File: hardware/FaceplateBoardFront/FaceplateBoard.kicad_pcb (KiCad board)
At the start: 2 copper layers, 33 x 66.5 mm, 20 parts, among them SW1 Mode_Encoder, SW2 Color_Encoder

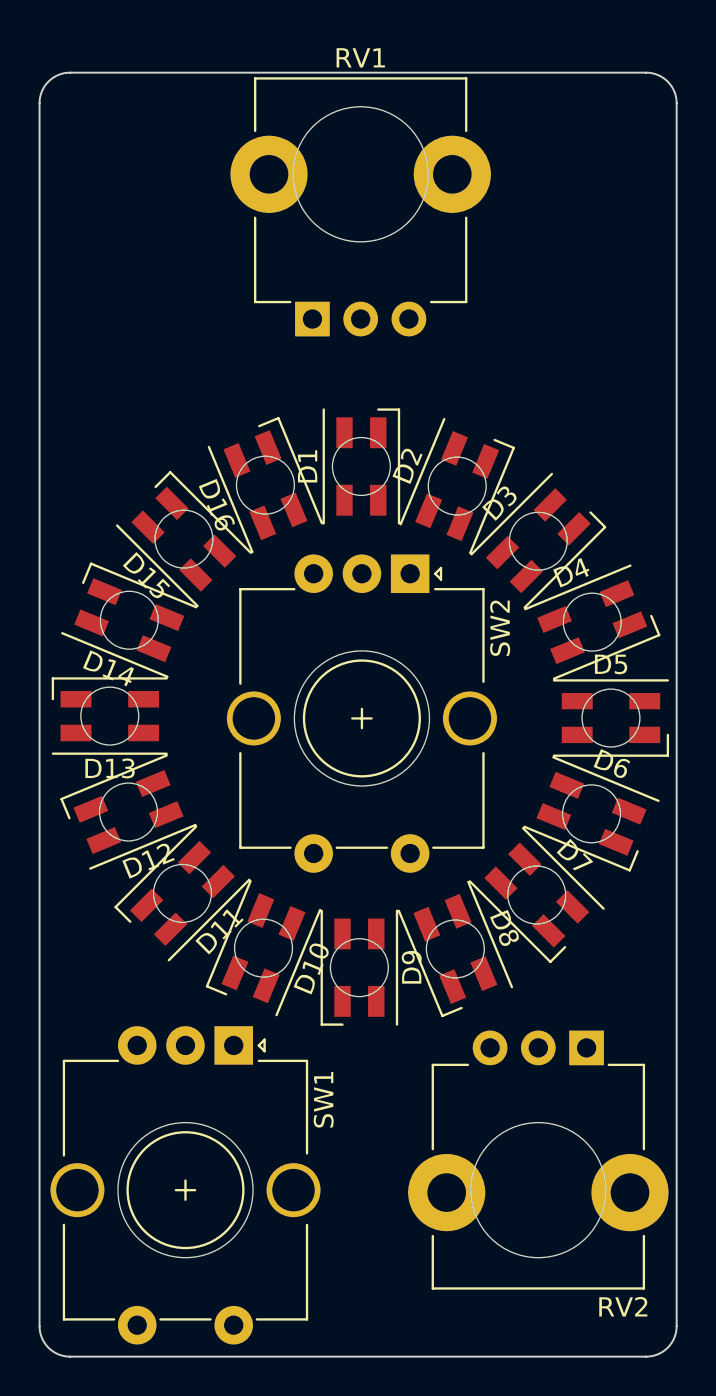
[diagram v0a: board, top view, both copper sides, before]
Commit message: After PCB v2
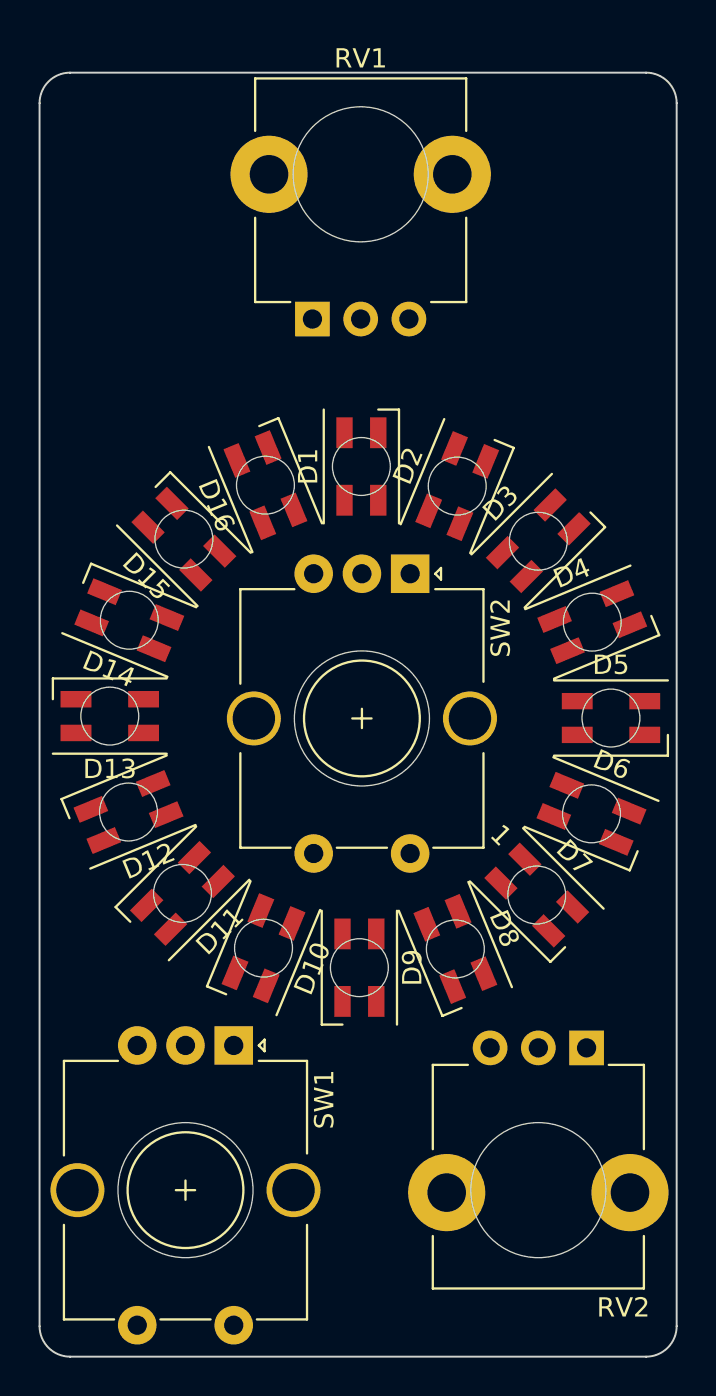
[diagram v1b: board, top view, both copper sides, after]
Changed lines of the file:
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@@
     (tags "LED RGB NeoPixel Mini")
     (attr smd)
-    (fp_text reference D16 (at 0 -2.75 112.5) (layer F.SilkS)
-      (effects (font (size 1 1) (thickness 0.15)))
-    )
-    (fp_text value WS2812B (at 0 3.25 112.5) (layer F.Fab)
+    (fp_text reference D16 (at 0.000001 -2.75 112.5) (layer F.SilkS)
+      (effects (font (size 1 1) (thickness 0.15)))
+    )
+    (fp_text value WS2812B (at 0 3.249999 112.5) (layer F.Fab)
       (effects (font (size 1 1) (thickness 0.15)))
     )
@@
     (tags "LED RGB NeoPixel Mini")
     (attr smd)
-    (fp_text reference D2 (at 0 -2.75 67.5) (layer F.SilkS)
-      (effects (font (size 1 1) (thickness 0.15)))
-    )
-    (fp_text value WS2812B (at 0 3.25 67.5) (layer F.Fab)
+    (fp_text reference D2 (at -0.000001 -2.75 67.5) (layer F.SilkS)
+      (effects (font (size 1 1) (thickness 0.15)))
+    )
+    (fp_text value WS2812B (at 0 3.249999 67.5) (layer F.Fab)
       (effects (font (size 1 1) (thickness 0.15)))
     )
@@
     (tags "LED RGB NeoPixel Mini")
     (attr smd)
-    (fp_text reference D14 (at 0 -2.75 157.5) (layer F.SilkS)
-      (effects (font (size 1 1) (thickness 0.15)))
-    )
-    (fp_text value WS2812B (at 0 3.25 157.5) (layer F.Fab)
+    (fp_text reference D14 (at -0.000001 -2.75 157.5) (layer F.SilkS)
+      (effects (font (size 1 1) (thickness 0.15)))
+    )
+    (fp_text value WS2812B (at 0 3.249999 157.5) (layer F.Fab)
       (effects (font (size 1 1) (thickness 0.15)))
     )
@@
     (tags "LED RGB NeoPixel Mini")
     (attr smd)
-    (fp_text reference D12 (at 0 -2.75 202.5) (layer F.SilkS)
-      (effects (font (size 1 1) (thickness 0.15)))
-    )
-    (fp_text value WS2812B (at 0 3.25 202.5) (layer F.Fab)
+    (fp_text reference D12 (at 0.000001 -2.75 202.5) (layer F.SilkS)
+      (effects (font (size 1 1) (thickness 0.15)))
+    )
+    (fp_text value WS2812B (at 0 3.249999 202.5) (layer F.Fab)
       (effects (font (size 1 1) (thickness 0.15)))
     )
@@
     (tags "LED RGB NeoPixel Mini")
     (attr smd)
-    (fp_text reference D10 (at 0 -2.75 247.5) (layer F.SilkS)
-      (effects (font (size 1 1) (thickness 0.15)))
-    )
-    (fp_text value WS2812B (at 0 3.25 247.5) (layer F.Fab)
+    (fp_text reference D10 (at -0.000001 -2.75 247.5) (layer F.SilkS)
+      (effects (font (size 1 1) (thickness 0.15)))
+    )
+    (fp_text value WS2812B (at 0 3.249999 247.5) (layer F.Fab)
       (effects (font (size 1 1) (thickness 0.15)))
     )
@@
     (tags "LED RGB NeoPixel Mini")
     (attr smd)
-    (fp_text reference D8 (at 0 -2.75 292.5) (layer F.SilkS)
-      (effects (font (size 1 1) (thickness 0.15)))
-    )
-    (fp_text value WS2812B (at 0 3.25 292.5) (layer F.Fab)
+    (fp_text reference D8 (at 0.000001 -2.75 292.5) (layer F.SilkS)
+      (effects (font (size 1 1) (thickness 0.15)))
+    )
+    (fp_text value WS2812B (at 0 3.249999 292.5) (layer F.Fab)
       (effects (font (size 1 1) (thickness 0.15)))
     )
@@
       (effects (font (size 0.5 0.5) (thickness 0.1)))
     )
+    (fp_text user 1 (at -3.5 -0.875 135) (layer F.SilkS)
+      (effects (font (size 1 1) (thickness 0.15)))
+    )
     (fp_text user e (at -3.5 -0.875 315) (layer F.SilkS) hide
       (effects (font (size 1 1) (thickness 0.15)))
@@
     (tags "LED RGB NeoPixel Mini")
     (attr smd)
-    (fp_text reference D6 (at 0 -2.75 337.5) (layer F.SilkS)
-      (effects (font (size 1 1) (thickness 0.15)))
-    )
-    (fp_text value WS2812B (at 0 3.25 337.5) (layer F.Fab)
+    (fp_text reference D6 (at -0.000001 -2.75 337.5) (layer F.SilkS)
+      (effects (font (size 1 1) (thickness 0.15)))
+    )
+    (fp_text value WS2812B (at 0 3.249999 337.5) (layer F.Fab)
       (effects (font (size 1 1) (thickness 0.15)))
     )
@@
     (tags "LED RGB NeoPixel Mini")
     (attr smd)
-    (fp_text reference D4 (at 0 -2.75 22.5) (layer F.SilkS)
-      (effects (font (size 1 1) (thickness 0.15)))
-    )
-    (fp_text value WS2812B (at 0 3.25 22.5) (layer F.Fab)
-      (effects (font (size 1 1) (thickness 0.15)))
-    )
+    (fp_text reference D4 (at 0.000001 -2.75 22.5) (layer F.SilkS)
+      (effects (font (size 1 1) (thickness 0.15)))
+    )
+    (fp_text value WS2812B (at 0 3.249999 22.5) (layer F.Fab)
+      (effects (font (size 1 1) (thickness 0.15)))
+    )
